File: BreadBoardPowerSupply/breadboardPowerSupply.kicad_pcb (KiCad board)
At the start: 2 copper layers, 31.2 x 53.5 mm, 18 parts, among them J1 Conn_01x02_Pin, J2 Conn_01x02_Pin, J3 Conn01x03Pin, J4 Conn_01x03_Pin, J5 Screw_Terminal_01x02, J6 Barrel_Jack_Switch, J7 Screw_Terminal_01x02, SW1 SW_Wuerth_450301014042, U1 LM7805_TO220, U2 LM317_TO-220

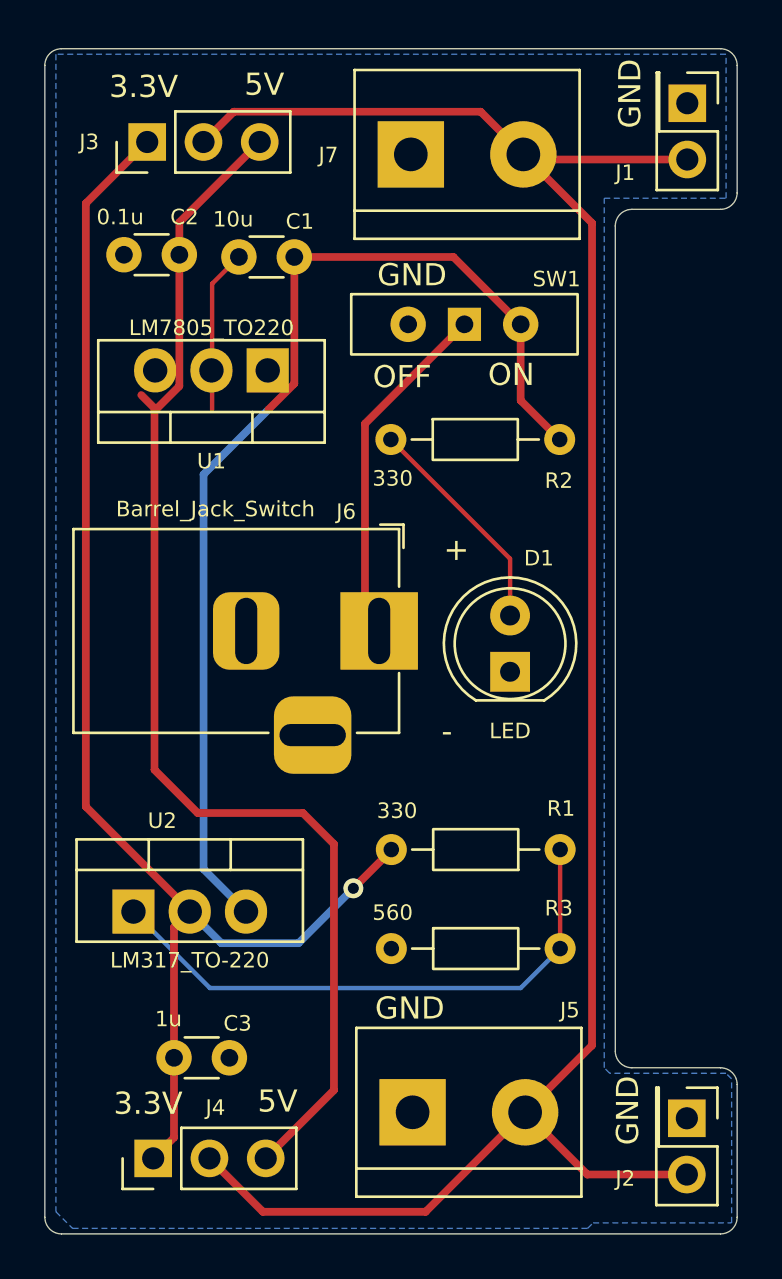
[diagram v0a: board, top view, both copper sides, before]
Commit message: Complete PCB
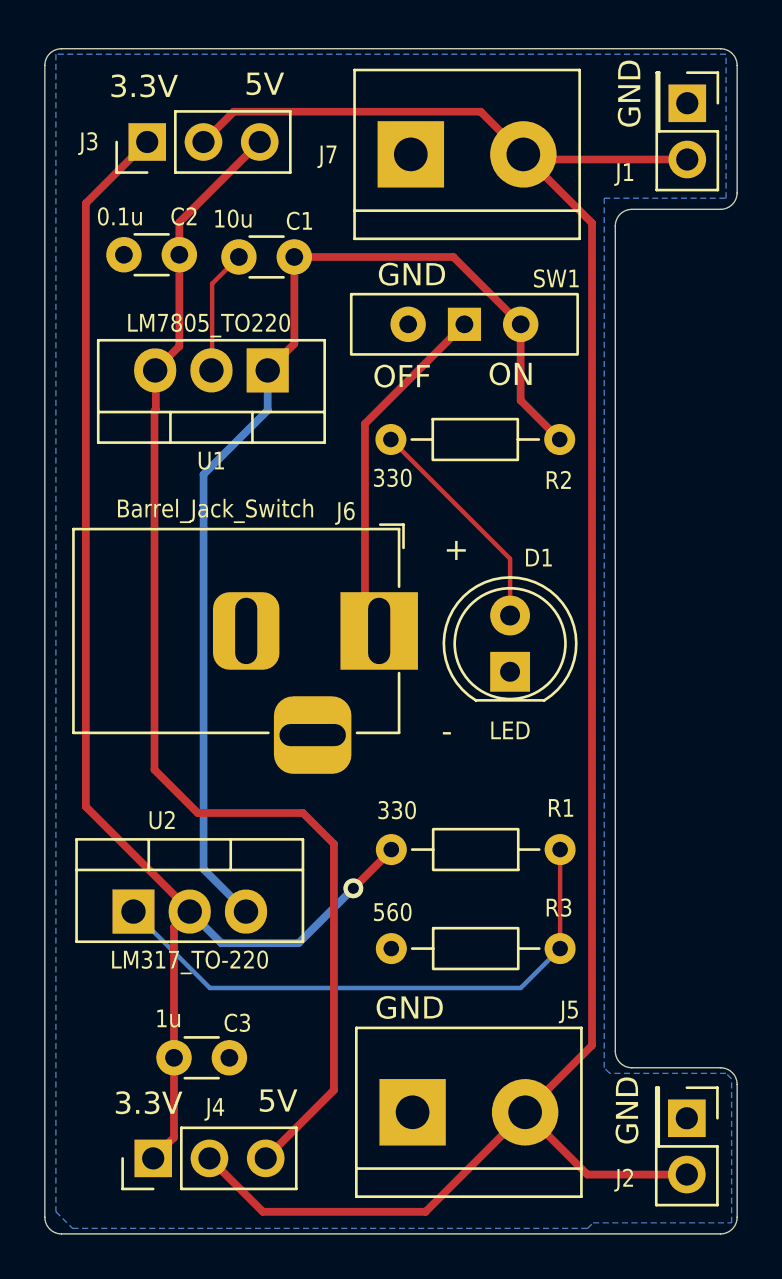
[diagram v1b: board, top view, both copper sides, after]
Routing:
- net GND: track 7.39 -> 5.63 mm
- net /5V: track 56.2 -> 55.3 mm
